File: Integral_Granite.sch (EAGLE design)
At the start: 34 parts, among them IC5 TLP785_GB,F_, IC6 TLP785_GB,F_, Q1 2SK4017_Q_, Q2 2SK4017_Q_

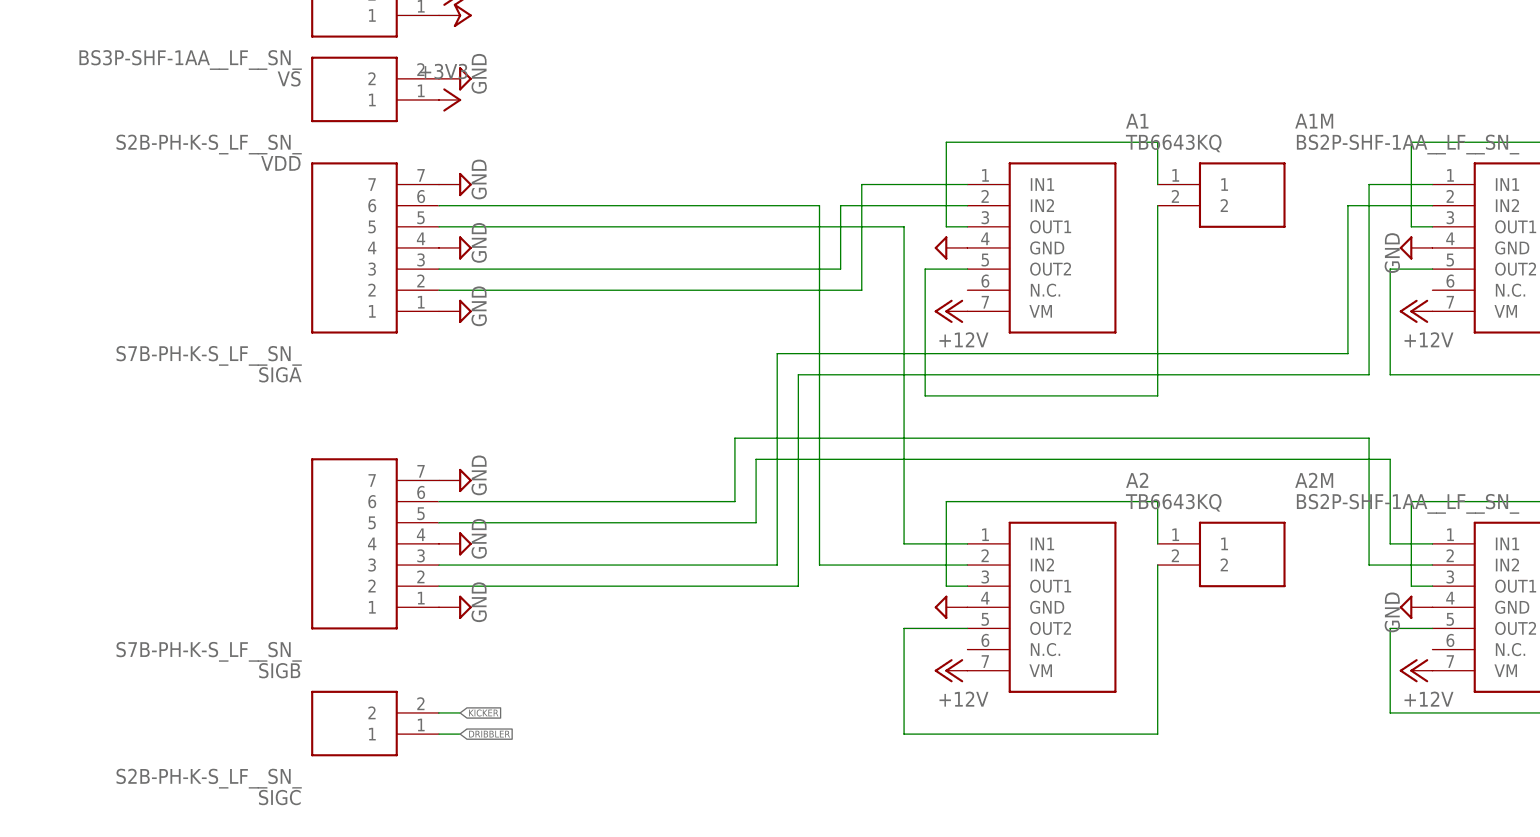
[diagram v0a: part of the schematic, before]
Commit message: initial commit
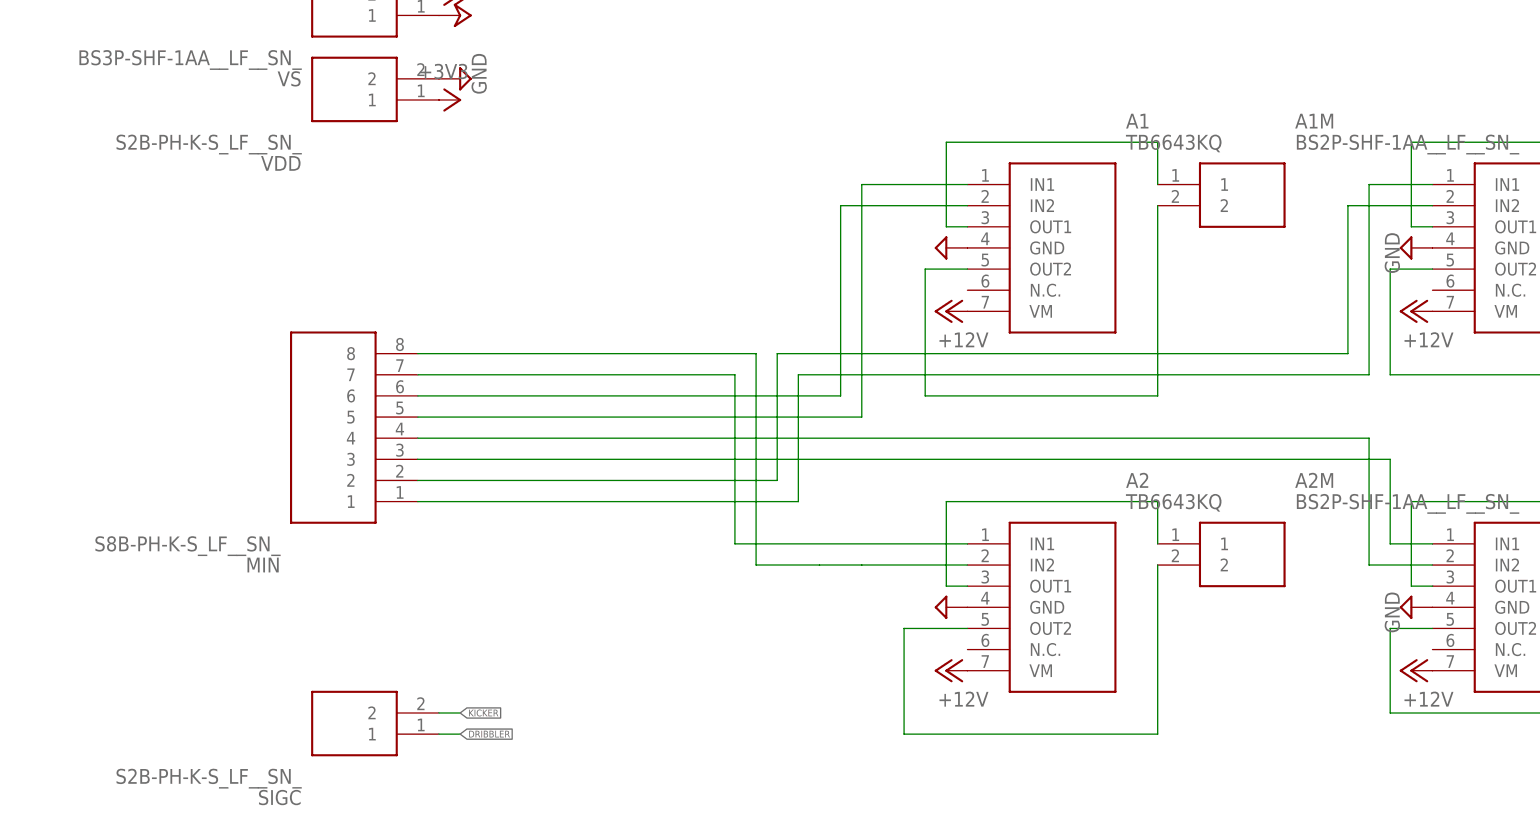
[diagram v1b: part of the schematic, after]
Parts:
- removed SIGA, SIGB: S7B-PH-K-S_LF__SN_, S7B-PH-K-S_LF__SN_:S7B-PH-K-S_LF__SN_
- added MIN: S8B-PH-K-S_LF__SN_, S8B-PH-K-S_LF__SN_:S8B-PH-K-S_LF__SN_
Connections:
- net GND: no longer SIGA.1, SIGA.4, SIGA.7, SIGB.1, SIGB.4, SIGB.7
- net N$1: now also MIN.5; no longer SIGA.2
- net N$2: now also MIN.6; no longer SIGA.3
- net N$3: now also MIN.7; no longer SIGA.5
- net N$4: now also MIN.8; no longer SIGA.6
- net N$5: now also MIN.1; no longer SIGB.2
- net N$6: now also MIN.2; no longer SIGB.3
- net N$7: now also MIN.3; no longer SIGB.5
- net N$8: now also MIN.4; no longer SIGB.6
